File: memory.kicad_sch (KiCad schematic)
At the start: 20 parts, among them J4 ALTRAM, U14 74LS32(ЛЛ1), U15 74LS74(ТМ2), U2 74LS20(ЛА1), U29 74LS257(КП11), U3 74LS04(ЛН1), U30 74LS257(КП11), U31 74LS257(КП11), U32 74LS257(КП11), U33 74LS257(КП11), U34 AS6C4008, U35 74LS245(АП6), U36 74LS670(ИР26), U37 74LS243(ИП7), U38 27C128, U4 74LS21(ЛИ6)

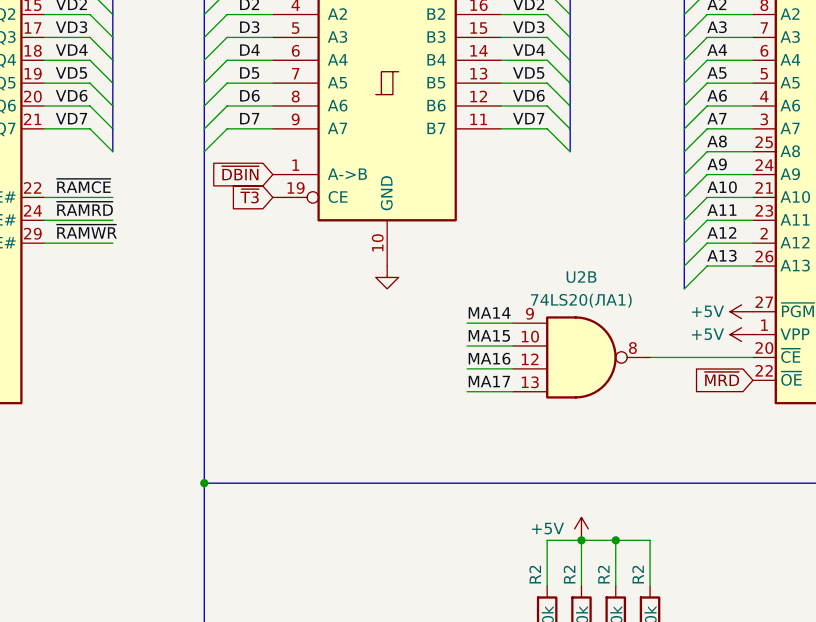
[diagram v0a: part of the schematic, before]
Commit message: fix RAM transceiver connections
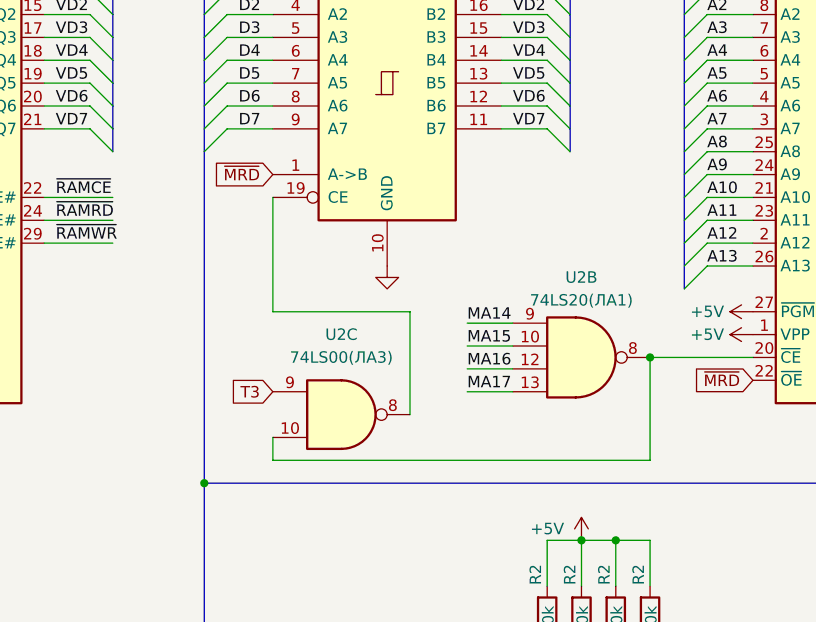
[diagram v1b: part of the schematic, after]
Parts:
- added unit 3 of U2
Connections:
- net ~{DBIN} is gone; now on net ~{MRD}: U35.1 (A->B)
- net T3: now also U2.9
- net at U2.8, U38.20 (~{CE}): now also U2.10
- net ~{T3}: no longer names the net of U35.19 (CE)
- net ~{T3}: now also U2.8
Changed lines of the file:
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@@
   (junction (at 173.99 133.35) (diameter 0) (color 0 0 0 0)
+  )
+  (junction (at 234.95 71.12) (diameter 0) (color 0 0 0 0)
   )
   (junction (at 231.14 91.44) (diameter 0) (color 0 0 0 0)
@@
     (stroke (width 0) (type default))
   )
+  (wire (pts (xy 208.28 66.04) (xy 208.28 77.47))
+    (stroke (width 0) (type default))
+  )
   (bus (pts (xy 238.76 38.1) (xy 238.76 40.64))
     (stroke (width 0) (type default))
@@
     (stroke (width 0) (type default))
   )
+  (wire (pts (xy 193.04 66.04) (xy 208.28 66.04))
+    (stroke (width 0) (type default))
+  )
   (wire (pts (xy 266.7 33.02) (xy 271.78 33.02))
     (stroke (width 0) (type default))
@@
     (stroke (width 0) (type default))
   )
+  (wire (pts (xy 234.95 82.55) (xy 234.95 71.12))
+    (stroke (width 0) (type default))
+  )
   (wire (pts (xy 104.14 54.61) (xy 96.52 54.61))
     (stroke (width 0) (type default))
@@
     (stroke (width 0) (type default))
   )
+  (wire (pts (xy 193.04 82.55) (xy 234.95 82.55))
+    (stroke (width 0) (type default))
+  )
   (wire (pts (xy 231.14 96.52) (xy 231.14 91.44))
     (stroke (width 0) (type default))
@@
     (stroke (width 0) (type default))
   )
+  (wire (pts (xy 193.04 80.01) (xy 193.04 82.55))
+    (stroke (width 0) (type default))
+  )
   (bus (pts (xy 185.42 35.56) (xy 185.42 33.02))
     (stroke (width 0) (type default))
@@
     (stroke (width 0) (type default))
   )
+  (wire (pts (xy 193.04 53.34) (xy 193.04 66.04))
+    (stroke (width 0) (type default))
+  )
   (bus (pts (xy 175.26 43.18) (xy 175.26 45.72))
     (stroke (width 0) (type default))
@@
   (label "D1" (at 189.23 30.48 0) (fields_autoplaced)
     (effects (font (size 1.27 1.27)) (justify left bottom))
-  )
-  (global_label "~{T3}" (shape input) (at 193.04 53.34 180) (fields_autoplaced)
-    (effects (font (size 1.27 1.27)) (justify right))
-    (property "Intersheetrefs" "${INTERSHEET_REFS}" (at 187.9571 53.34 0)
-      (effects (font (size 1.27 1.27)) (justify right) hide)
-    )
   )
   (global_label "T3" (shape input) (at 31.75 115.57 180) (fields_autoplaced)
@@
     )
   )
+  (global_label "T3" (shape input) (at 193.04 74.93 180) (fields_autoplaced)
+    (effects (font (size 1.27 1.27)) (justify right))
+    (property "Intersheetrefs" "${INTERSHEET_REFS}" (at 187.8777 74.93 0)
+      (effects (font (size 1.27 1.27)) (justify right) hide)
+    )
+  )
   (global_label "VA15" (shape input) (at 78.74 140.97 180) (fields_autoplaced)
     (effects (font (size 1.27 1.27)) (justify right))
@@
     )
   )
+  (global_label "~{MRD}" (shape input) (at 193.04 50.8 180) (fields_autoplaced)
+    (effects (font (size 1.27 1.27)) (justify right))
+    (property "Intersheetrefs" "${INTERSHEET_REFS}" (at 186.1428 50.8 0)
+      (effects (font (size 1.27 1.27)) (justify right) hide)
+    )
+  )
   (global_label "T3" (shape input) (at 25.4 58.42 180) (fields_autoplaced)
     (effects (font (size 1.27 1.27)) (justify right))
     (property "Intersheetrefs" "${INTERSHEET_REFS}" (at 20.2377 58.42 0)
-      (effects (font (size 1.27 1.27)) (justify right) hide)
-    )
-  )
-  (global_label "~{DBIN}" (shape input) (at 193.04 50.8 180) (fields_autoplaced)
-    (effects (font (size 1.27 1.27)) (justify right))
-    (property "Intersheetrefs" "${INTERSHEET_REFS}" (at 185.6589 50.8 0)
       (effects (font (size 1.27 1.27)) (justify right) hide)
     )
@@
         )
       )
+    )
+  )
+  (symbol (lib_id "74xx:74LS00") (at 200.66 77.47 0) (unit 3)
+    (in_bom yes) (on_board yes) (dnp no)
+    (property "Reference" "U2" (at 200.6517 68.58 0)
+      (effects (font (size 1.27 1.27)))
+    )
+    (property "Value" "74LS00(ЛА3)" (at 200.6517 71.12 0)
+      (effects (font (size 1.27 1.27)))
+    )
+    (property "Footprint" "Package_DIP:DIP-14_W7.62mm" (at 200.66 77.47 0)
+      (effects (font (size 1.27 1.27)) hide)
+    )
+    (property "Datasheet" "http://www.ti.com/lit/gpn/sn74ls00" (at 200.66 77.47 0)
+      (effects (font (size 1.27 1.27)) hide)
+    )
+    (pin "1")
+    (pin "2")
+    (pin "3")
+    (pin "4")
+    (pin "5")
+    (pin "6")
+    (pin "10")
+    (pin "8")
+    (pin "9")
+    (pin "11")
+    (pin "12")
+    (pin "13")
+    (pin "14")
+    (pin "7")
+    (instances
+      (project "pac80"
+        (path "/76485272-58b9-4241-940e-8879fa844c96/e5b989ce-1e05-4470-9bcf-aea14f9cddaf"
+          (reference "U2") (unit 3)
+        )
+        (path "/76485272-58b9-4241-940e-8879fa844c96/3455005e-76fb-4d3b-af2a-bae2cb5cdaf9"
+          (reference "U2") (unit 3)
+        )
+        (path "/76485272-58b9-4241-940e-8879fa844c96/34cd57db-2a21-4ed7-a0b6-b6a247ac7439"
+          (reference "U2") (unit 3)
+        )
+        (path "/76485272-58b9-4241-940e-8879fa844c96/0567776f-ec27-40d8-a046-f38d0368ad09"
+          (reference "U2") (unit 3)
+        )
+      )
